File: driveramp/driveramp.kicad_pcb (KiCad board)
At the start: 2 copper layers, 109 x 79 mm, 86 parts, among them J1 SMA, J2 SMA, K1 CONN_3, K2 CONN_3, P2 CONN_2, Q1 BC547BTA, T1 MABACT0067, T2 2x Fair-Rite 2843006802, coax, U1 ISL43210A, U2 MRFE6VP100H, U3 LM317HV, U4 7321MF, U5 GALI6+, U6 BA08CC0WFP

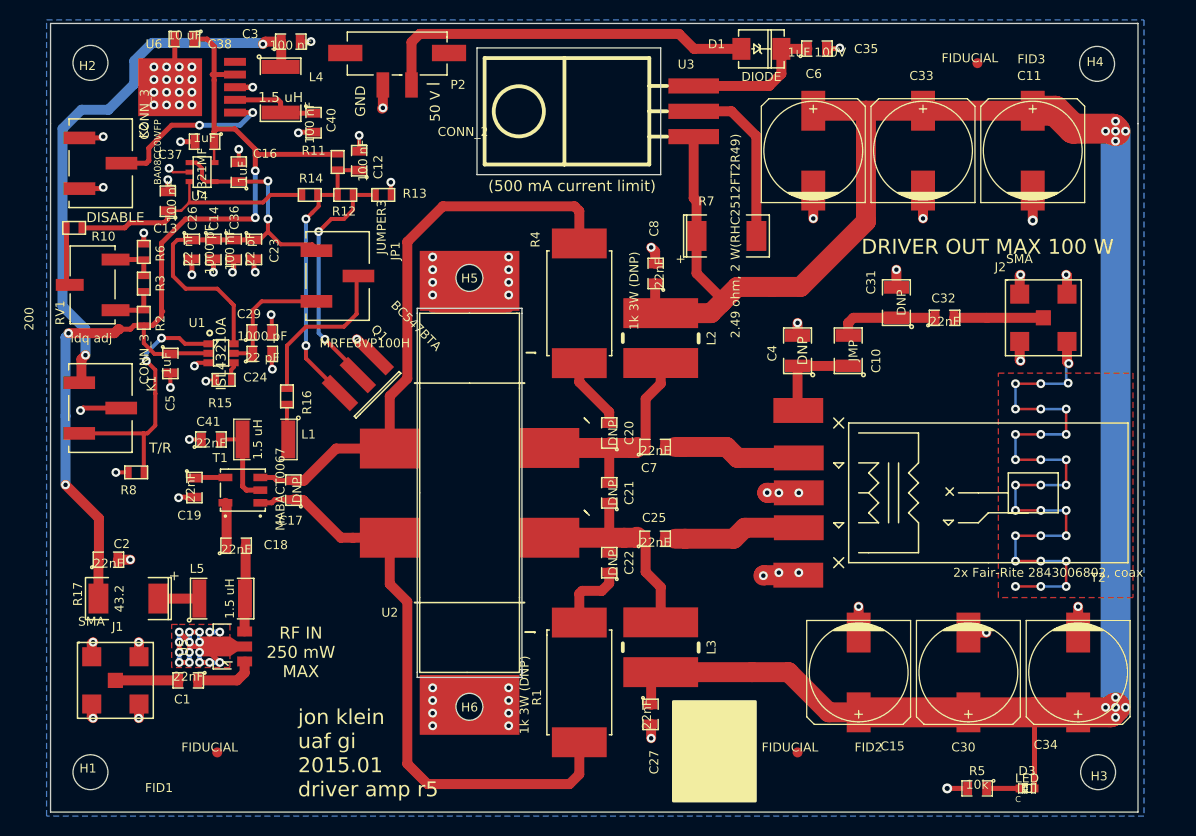
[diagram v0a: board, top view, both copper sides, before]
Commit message: DFM changes..
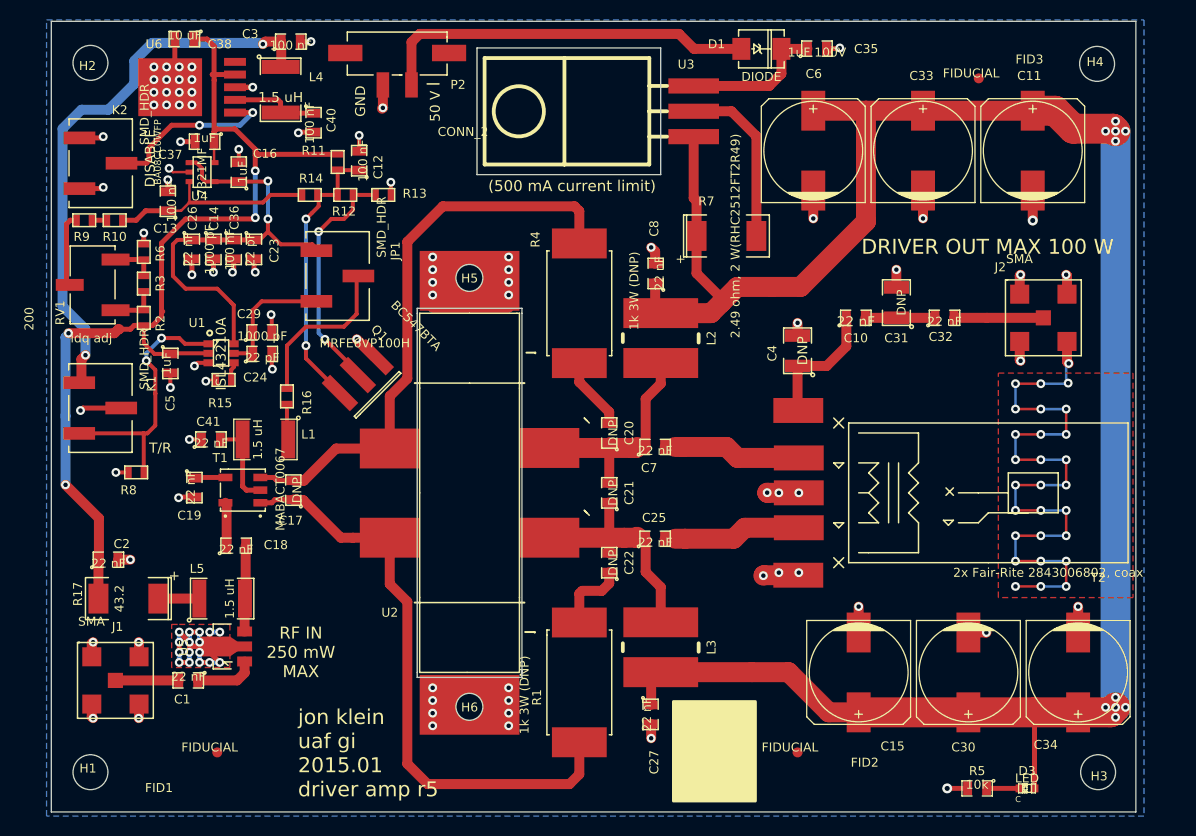
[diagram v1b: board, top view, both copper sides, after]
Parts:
- added R9: 1.1k 1%, SMD_Packages:SMD-0603, F.Cu at (79.4, 82.7)
- C1, C18, C19, C2, C25, C27, C32, C41, C7, C8: value 22nF -> 22 nF
- C10: value JMP -> 22 nF; footprint SMD_Packages:SMD-1210 -> SMD_Packages:SMD-0805
- JP1: value JUMPER3 -> SMD_HDR
- K1, K2: value CONN_3 -> SMD_HDR
- R10: value 2k 1% -> 909 1%
- moved R10 4.13 mm to (82.4, 82.7), turned to 0 degrees
- moved C10 3.39 mm to (156.7, 92.5), turned to 0 degrees
- moved FID3 1.53 mm to (169.0, 68.5)
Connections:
- R10 pad 1: Net-(C13-Pad1) -> Net-(R10-Pad1)
- R10 pad 2: Net-(R10-Pad2) -> Net-(C13-Pad1)
- RV1 pad 2: Net-(R10-Pad2) -> Net-(R9-Pad1)
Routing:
- net Net-(R9-Pad1): track 0.00 -> 7.41 mm
- net Net-(R10-Pad2): track 5.85 -> 0.00 mm
- net Net-(C13-Pad1): track 26.0 -> 21.2 mm
- net Net-(C10-Pad1): track 9.75 -> 13.2 mm
- net Net-(C10-Pad2): track 10.2 -> 6.98 mm
- net Net-(R10-Pad1): track 0.00 -> 1.52 mm
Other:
- board size 109 x 79 mm -> 108.7 x 79.2 mm
